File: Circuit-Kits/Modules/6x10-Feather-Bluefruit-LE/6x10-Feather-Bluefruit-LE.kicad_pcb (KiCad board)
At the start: 2 copper layers, 47.8 x 79.8 mm, 2 parts, among them U1 ADAFRUIT-FEATHER-BLUEFRUIT-LE

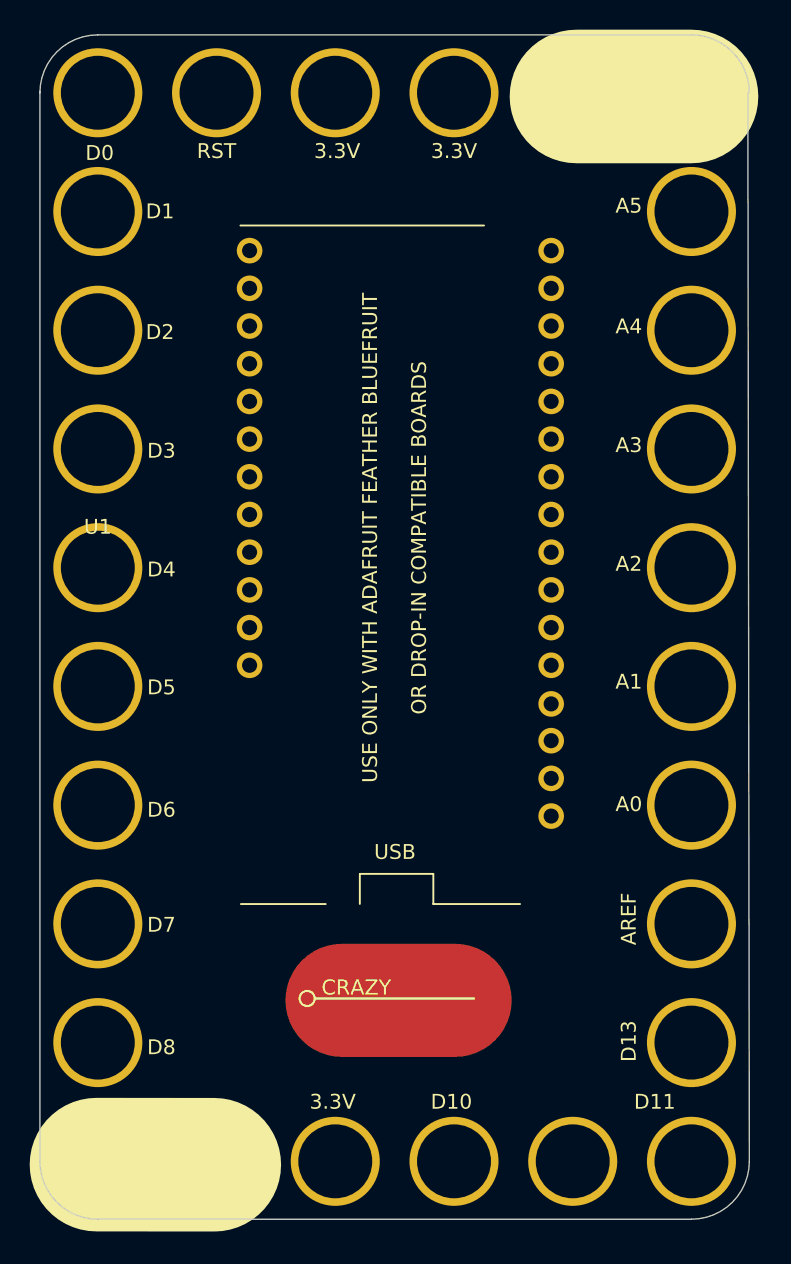
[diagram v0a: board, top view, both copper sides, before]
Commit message: Release v1.0 Adafruit Feather Bluefruit Breakout
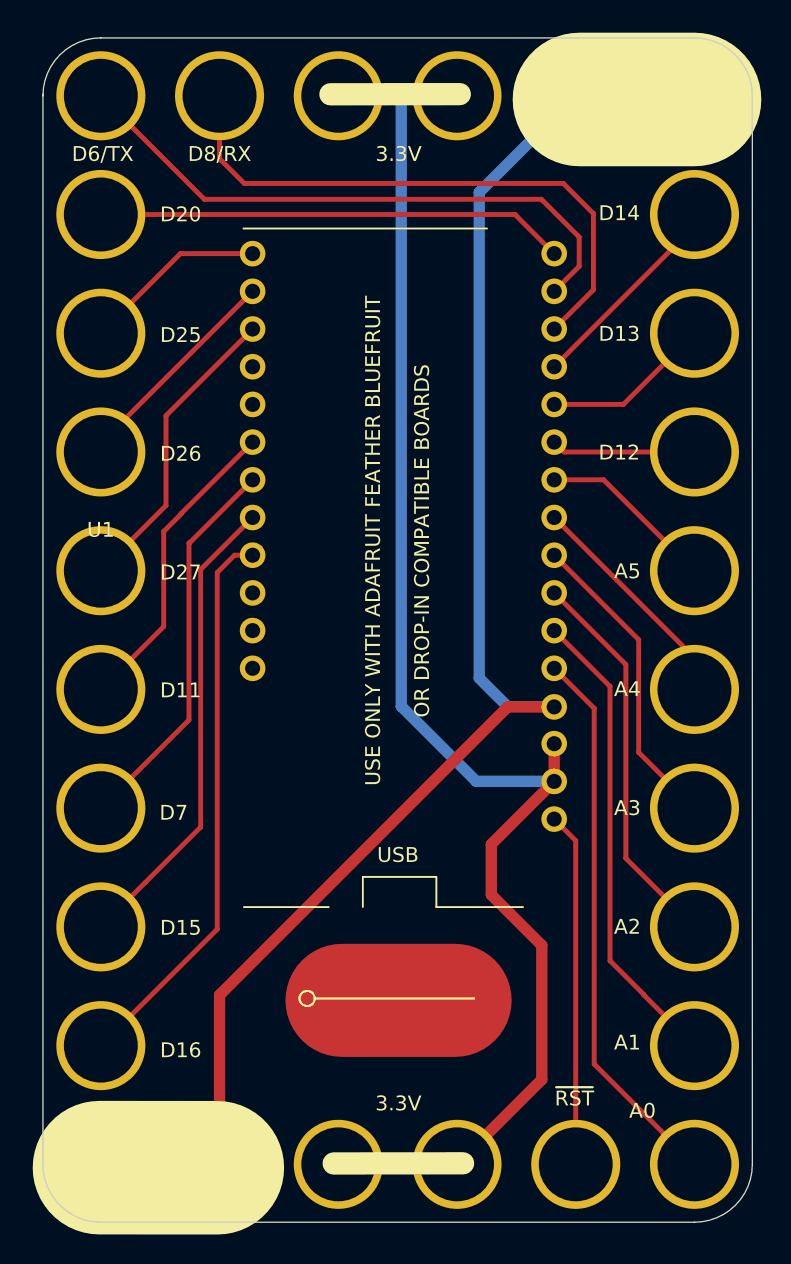
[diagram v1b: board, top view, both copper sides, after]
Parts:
- moved U1 0.29 mm to (27.4, 58.7)
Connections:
- U1 pad 15: (no net) -> /A0
- U1 pad 16: (no net) -> /A1
- U1 pad 17: (no net) -> /A2
- U1 pad 18: (no net) -> /A3
- U1 pad 19: (no net) -> /D6_TX
- U1 pad 2: (no net) -> /D25
- U1 pad 20: (no net) -> /D7
- U1 pad 21: (no net) -> /D8_RX
- U1 pad 25: (no net) -> /D11
- U1 pad 26: (no net) -> /D12_SCK
- U1 pad 27: (no net) -> /D13_MOSI
- U1 pad 28: (no net) -> /D14_MISO
- U1 pad 29: (no net) -> /D15
- U1 pad 3: (no net) -> /D27
- U1 pad 30: (no net) -> /D16
- U1 pad 34: (no net) -> /D20_DFU
- U1 pad 4: (no net) -> /D26
- U1 pad 5: (no net) -> /A4
- U1 pad 6: (no net) -> /A5
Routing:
- net GND: track 0.00 -> 105.8 mm
- net VCC: track 0.00 -> 103.4 mm
- net /D6_TX: track 0.00 -> 40.5 mm
- net /D8_RX: track 0.00 -> 39.8 mm
- net /D16: track 0.00 -> 38.0 mm
- net /A0: track 0.00 -> 37.3 mm
- net /A1: track 0.00 -> 31.9 mm
- net /D15: track 0.00 -> 31.8 mm
- net /D20_DFU: track 0.00 -> 31.6 mm
- net /A2: track 0.00 -> 26.4 mm
- net /D7: track 0.00 -> 26.4 mm
- net /~RST: track 0.00 -> 23.9 mm
- net /A3: track 0.00 -> 21.0 mm
- net /D11: track 0.00 -> 20.9 mm
- net /D26: track 0.00 -> 20.5 mm
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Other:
- outline, holes or cut-outs redrawn
- board text added: "CIRCUITS"
- board text added: "FABRICATION NOTES 1. THIS IS A 2 LAYER BOARD. 2. EXTERNAL LAYERS SHALL HAVE 1 OZ COPPER. 3. MATERIAL: FR4 AND 0.062 INCH +/- 10% THICK. 4. BOARDS SHALL BE ROHS COMPLIANT. 5. MANUFACTURE IN ACCORDANCE WITH IPC-6012 CLASS 2 6. MASK: BOTH SIDES OF THE BOARD SHALL HAVE SOLDER MASK (GREEN) OVER BARE COPPER. 7. SILK: BOTH SIDES OF THE BOARD SHALL HAVE WHITE SILKSCREEN. DO NOT PLACE SILK OVER BARE COPPE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"
- board text removed: "FABRICATION NOTES 1. THIS IS A 2 LAYER BOARD. 2. EXTERNAL LAYERS SHALL HAVE 1 OZ COPPER. 3. MATERIAL: FR4 AND 0.062 INCH +/- 10% THICK. 4. BOARDS SHALL BE ROHS COMPLIANT. 5. MANUFACTURE IN ACCORDANCE WITH IPC-6012 CLASS 2 6. MASK: BOTH SIDES OF THE BOARD SHALL HAVE SOLDER MASK (ANY COLOR) OVER BARE COPPER. 7. SILK: BOTH SIDES OF THE BOARD SHALL HAVE WHITE SILKSCREEN. DO NOT PLACE SILK OVER BARE C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"
